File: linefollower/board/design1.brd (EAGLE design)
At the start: 44 parts, among them IC1 STM32F10XCXT6, IC2 FT232RL, Q1 8mhz, Q2 32khz, X1 MINI-USB-32005-201

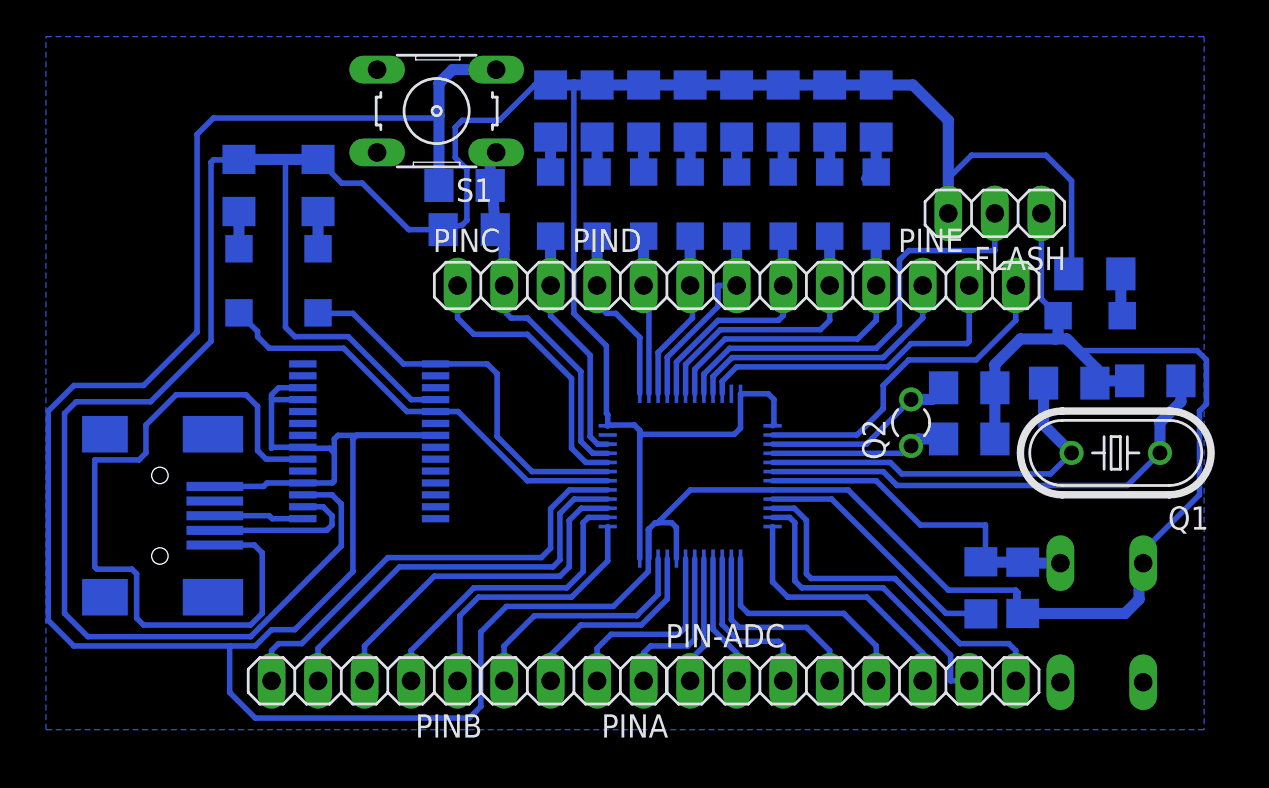
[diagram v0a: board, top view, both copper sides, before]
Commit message: revisi board
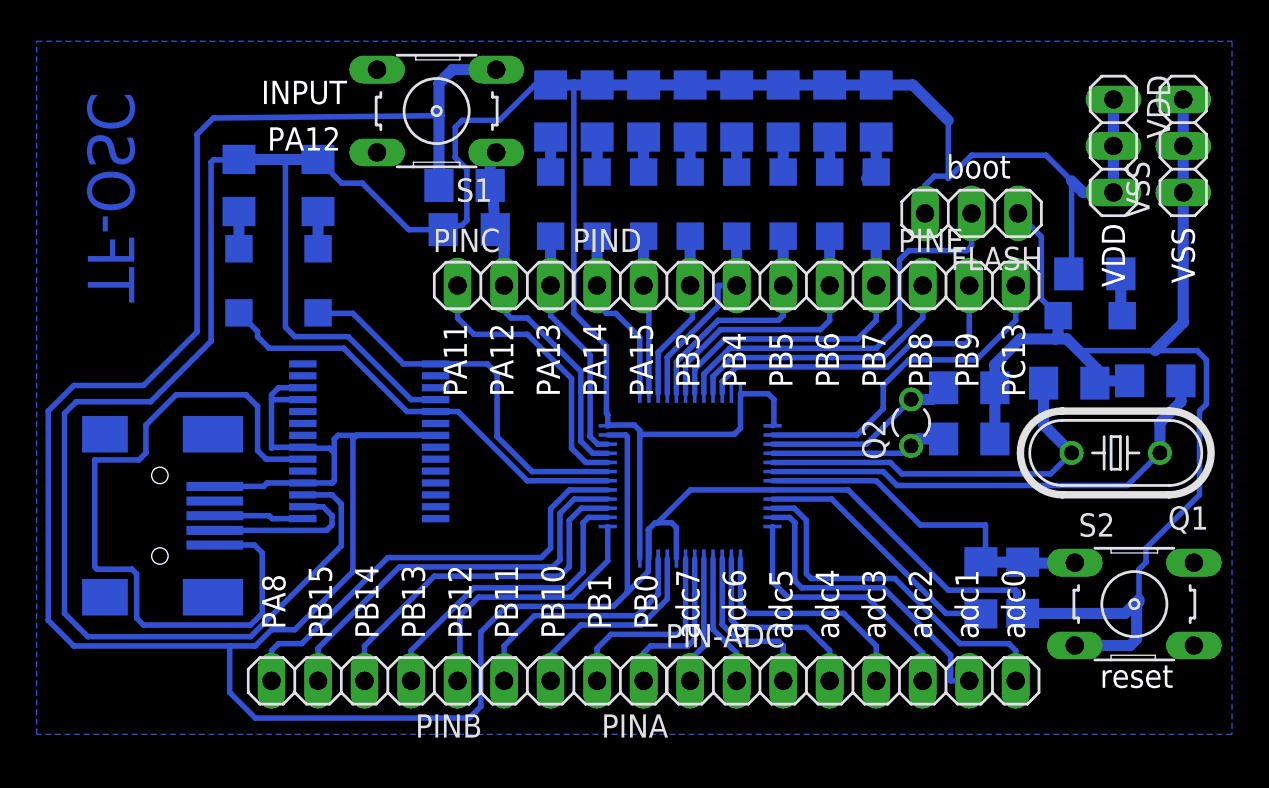
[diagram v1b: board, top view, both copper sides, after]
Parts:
- added VDD, VSS: (no value), pinhead:1X03
- moved S2 2.05 mm to (72.5, 41.0), flipped to the top, turned to 0 degrees
- moved FLASH 1.27 mm to (63.6, 62.4)
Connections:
- net N$1 renamed ADC7
- net N$2 renamed ADC6
- net N$3 renamed ADC5
- net N$4 renamed ADC4
- net N$5 renamed ADC3
- net N$6 renamed ADC2
- net N$7 renamed ADC1
- net N$8 renamed ADC0
- net VDD: now also VDD.1, VDD.2, VDD.3
- net VSS: now also VSS.1, VSS.2, VSS.3
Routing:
- net VSS: track 234.0 -> 262.0 mm
- net VDD: track 194.6 -> 201.4 mm
- net N$13: track 23.9 -> 22.5 mm
- net NRST: track 19.1 -> 19.9 mm
- added copper zone on layer 16, net N$1
- removed copper zone on layer 16, net N$25
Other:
- board text added: "INPUT PA12"
- board text added: "PA11 PA12 PA13 PA14 PA15 PB3 PB4 PB5 PB6 PB7 PB8 PB9 PC13"
- board text added: "PA8 PB15 PB14 PB13 PB12 PB11 PB10 PB1 PB0"
- board text added: "TF-OSC"
- board text added: "VDD"
- board text added: "VSS"
- board text added: "adc7 adc6 adc5 adc4 adc3 adc2 adc1 adc0"
- board text added: "boot"
- board text added: "reset"
